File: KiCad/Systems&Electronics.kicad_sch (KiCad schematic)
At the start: 22 parts, among them U1 HX711, U3 MAX485E, U4 MAX485E

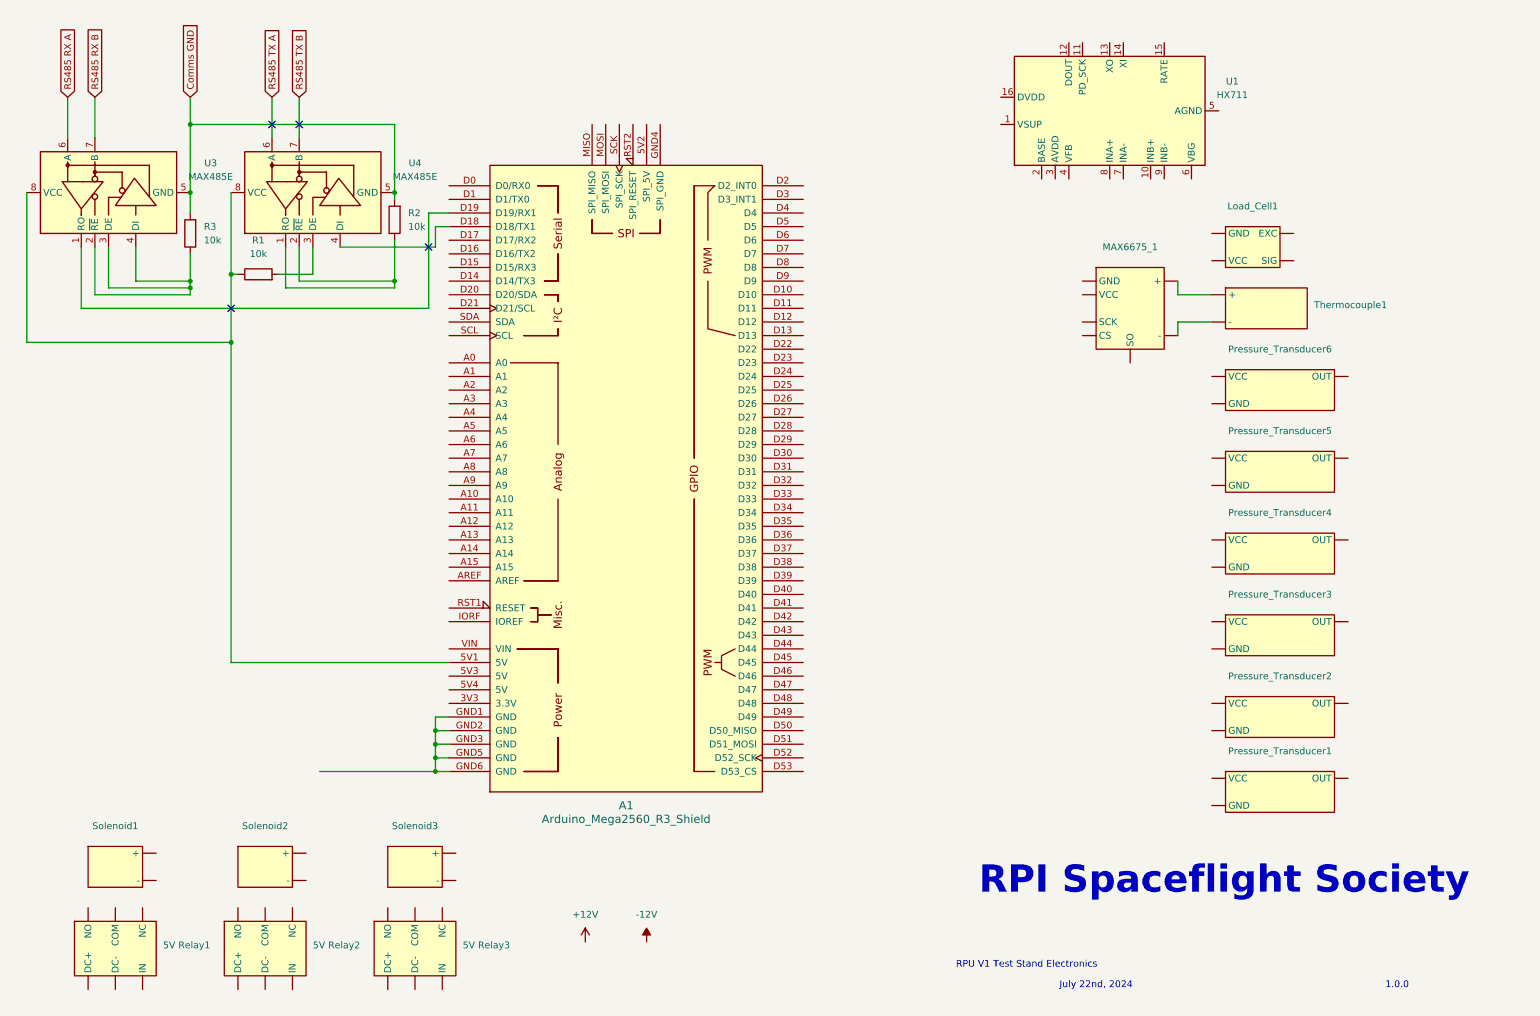
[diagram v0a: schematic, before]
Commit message: V1 Systems Schematics
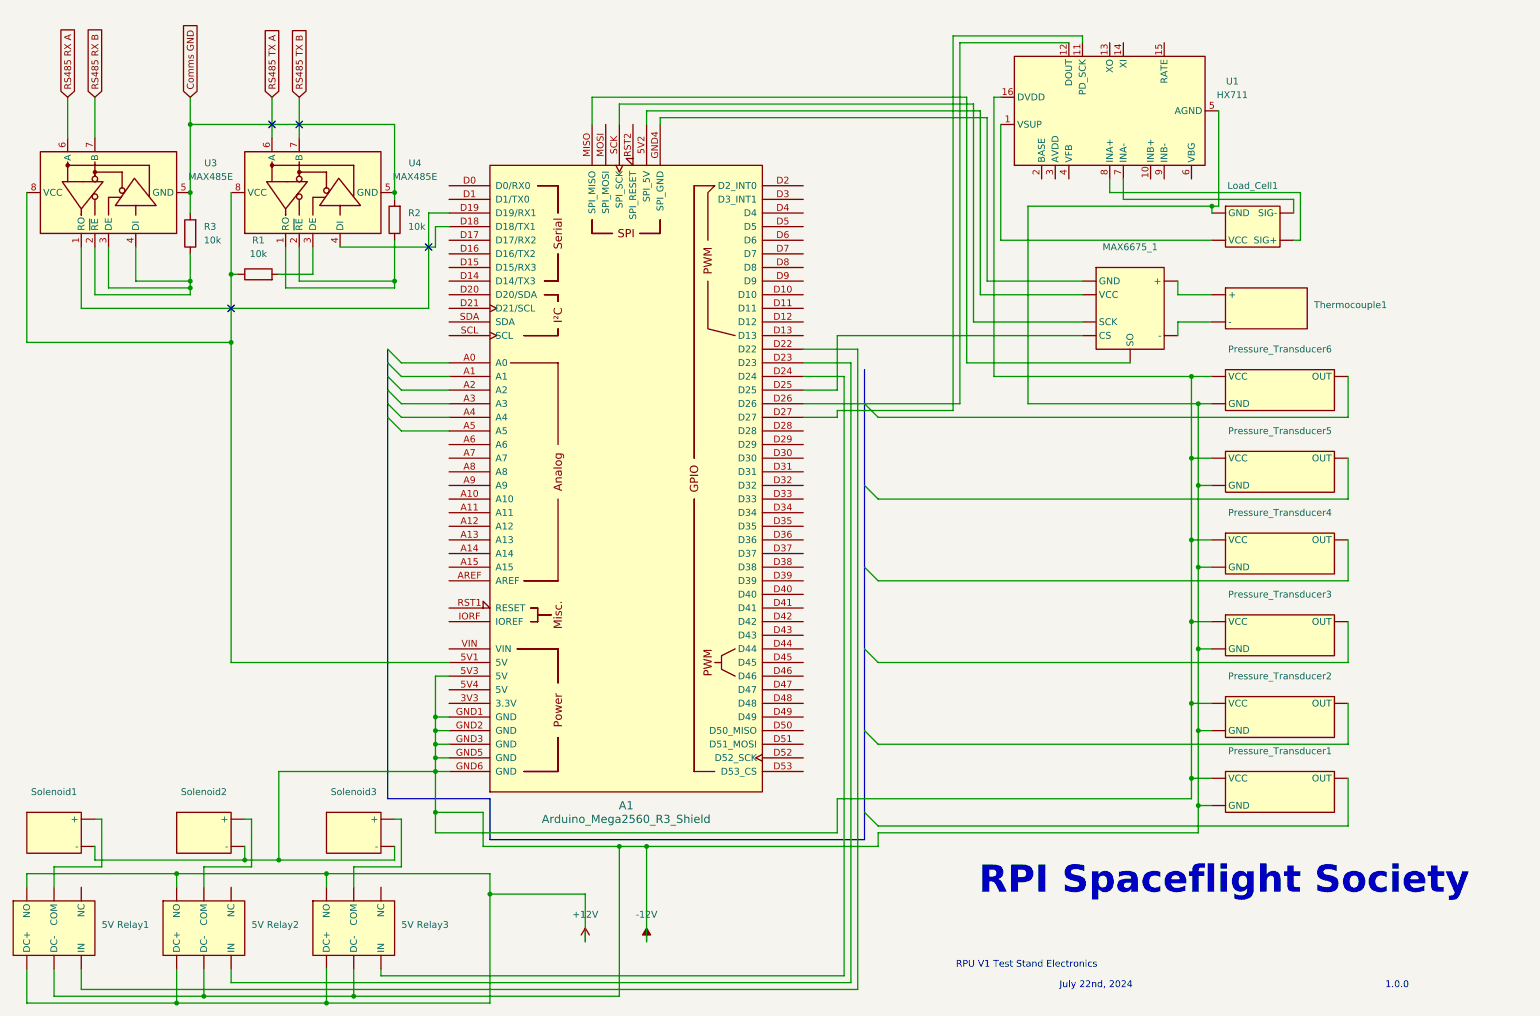
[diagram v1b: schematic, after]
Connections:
- net +12V: now also 5V Relay1. (NO), 5V Relay2. (NO), 5V Relay3. (NO)
- net -12V: now also 5V Relay1. (NO), 5V Relay2. (NO), 5V Relay3. (NO), A1.5V3 (5V), A1.GND1 (GND), A1.GND2 (GND), A1.GND3 (GND), A1.GND5 (GND), A1.GND6 (GND), Load_Cell1. (VCC), Pressure_Transducer1. (VCC), Pressure_Transducer2. (VCC), Pressure_Transducer3. (VCC), Pressure_Transducer4. (VCC), Pressure_Transducer5. (VCC), Pressure_Transducer6. (VCC), Solenoid1. (-), Solenoid2. (-), Solenoid3. (-), U1.16 (DVDD), U1.5 (AGND)
- net at A1.5V2 (SPI_5V): now also MAX6675_1. (VCC)
- net at A1.D22: now also 5V Relay1. (NO)
- net at A1.D23: now also 5V Relay2. (NO)
- net at A1.D24: now also 5V Relay3. (NO)
- net at A1.D25: now also MAX6675_1. (VCC)
- net at A1.D26: now also U1.12 (DOUT)
- net at A1.D27: now also U1.11 (PD_SCK)
- net at A1.GND4 (SPI_GND): now also MAX6675_1. (VCC)
- net at A1.MISO (SPI_MISO): now also MAX6675_1. (VCC)
- net at A1.SCK (SPI_SCK): now also MAX6675_1. (VCC)
- net at MAX6675_1. (VCC): now also Thermocouple1. (-)
- net at U1.1 (VSUP): now also Load_Cell1. (VCC)
- net at U1.7 (INA-): now also Load_Cell1. (VCC)
- net at U1.8 (INA+): now also Load_Cell1. (VCC)
- new net: 5V Relay1. (NO), Solenoid1. (-)
- new net: 5V Relay3. (NO), Solenoid3. (-)
- new net: 5V Relay2. (NO), Solenoid2. (-)
- new net: MAX6675_1. (VCC), Thermocouple1. (-)
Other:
- moved on the sheet: 5V Relay1, 5V Relay2, 5V Relay3, Solenoid1, Solenoid2, Solenoid3

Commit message: Electronics Schematic V1.1.0
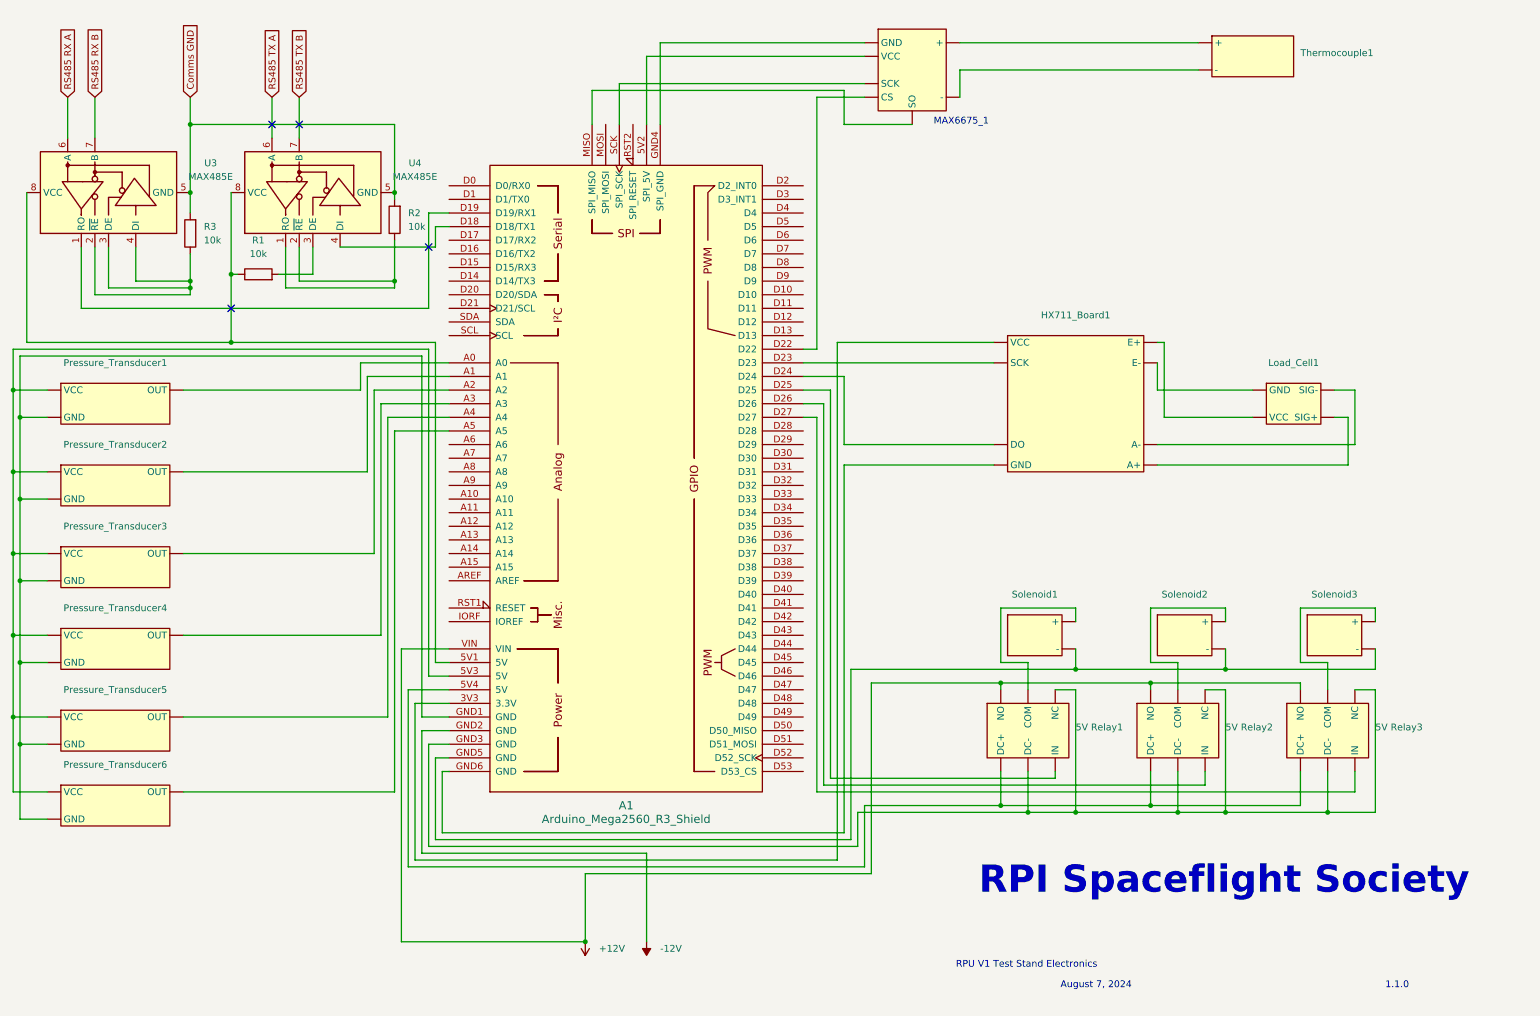
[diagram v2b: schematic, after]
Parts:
- removed U1: HX711, Package_SO:SOP-16_3.9x9.9mm_P1.27mm, symbol Analog_ADC:HX711
- added HX711_Board1: ~, symbol Sensors:HX711_Board
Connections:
- net +12V: now also A1.VIN
- net -12V: no longer 5V Relay1. (NO), 5V Relay2. (NO), 5V Relay3. (NO), A1.5V3 (5V), A1.GND1 (GND), A1.GND3 (GND), A1.GND5 (GND), A1.GND6 (GND), Load_Cell1. (VCC), Pressure_Transducer1. (VCC), Pressure_Transducer2. (VCC), Pressure_Transducer3. (VCC), Pressure_Transducer4. (VCC), Pressure_Transducer5. (VCC), Pressure_Transducer6. (VCC), Solenoid1. (-), Solenoid2. (-), Solenoid3. (-)
- net at A1.D22: now also MAX6675_1. (VCC); no longer 5V Relay1. (NO)
- net at Solenoid1. (-): now also A1.GND5 (GND), Solenoid2. (-), Solenoid3. (-); no longer 5V Relay1. (NO)
- net at A1.3V3 (3.3V): now also HX711_Board1. (VCC)
- net at A1.5V4 (5V): now also 5V Relay1. (NO), 5V Relay2. (NO), 5V Relay3. (NO)
- net at A1.A0: now also Pressure_Transducer1. (VCC)
- net at A1.A1: now also Pressure_Transducer2. (VCC)
- net at A1.A2: now also Pressure_Transducer3. (VCC)
- net at A1.A3: now also Pressure_Transducer4. (VCC)
- net at A1.A4: now also Pressure_Transducer5. (VCC)
- net at A1.A5: now also Pressure_Transducer6. (VCC)
- net at A1.D23: now also HX711_Board1. (VCC); no longer 5V Relay2. (NO)
- net at A1.D24: now also HX711_Board1. (VCC); no longer 5V Relay3. (NO)
- net at A1.D25: now also 5V Relay1. (NO); no longer MAX6675_1. (VCC)
- net at A1.D26: now also 5V Relay2. (NO)
- net at A1.D27: now also 5V Relay3. (NO)
- net at Pressure_Transducer2. (VCC): now also A1.GND1 (GND), Pressure_Transducer1. (VCC), Pressure_Transducer3. (VCC), Pressure_Transducer4. (VCC), Pressure_Transducer5. (VCC), Pressure_Transducer6. (VCC)
- net at Load_Cell1. (VCC): now also HX711_Board1. (VCC)
- new net: 5V Relay1. (NO), 5V Relay2. (NO), 5V Relay3. (NO), A1.GND3 (GND)
- new net: 5V Relay1. (NO), Solenoid1. (-)
- new net: A1.5V3 (5V), Pressure_Transducer1. (VCC), Pressure_Transducer2. (VCC), Pressure_Transducer3. (VCC), Pressure_Transducer4. (VCC), Pressure_Transducer5. (VCC), Pressure_Transducer6. (VCC)
- new net: A1.GND6 (GND), HX711_Board1. (VCC)
- new net: HX711_Board1. (VCC), Load_Cell1. (VCC) (x3)
- new net: MAX6675_1. (VCC), Thermocouple1. (-)
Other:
- note added: "1.1.0"
- note added: "August 7, 2024"
- note added: "MAX6675_1"
- note removed: "1.0.0"
- note removed: "July 22nd, 2024"
- moved on the sheet: 5V Relay1, 5V Relay2, 5V Relay3, Load_Cell1, Solenoid1, Solenoid2, Solenoid3, Thermocouple1
